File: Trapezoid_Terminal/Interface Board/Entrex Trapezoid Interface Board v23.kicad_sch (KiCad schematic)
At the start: 103 parts, among them P15 Conn_02x40_Odd_Even_Shielded, SW1 SW_DIP_x08

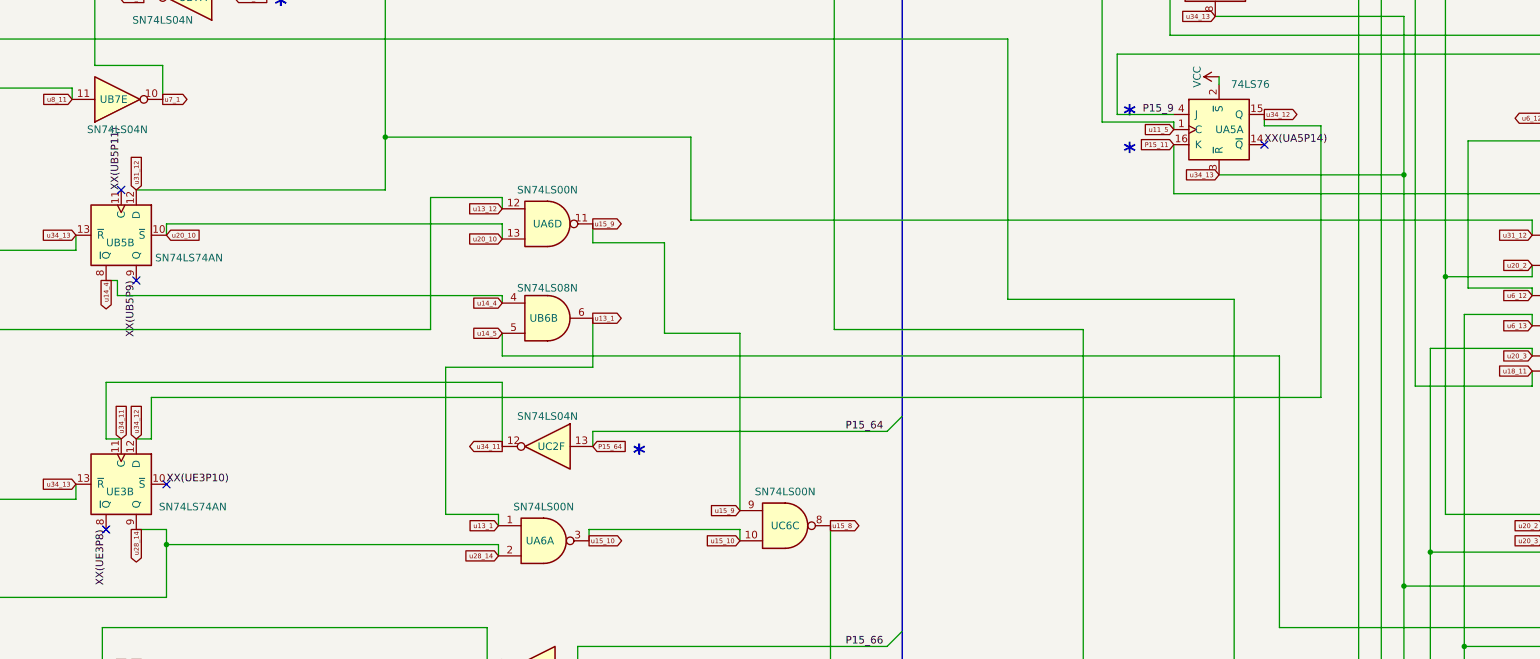
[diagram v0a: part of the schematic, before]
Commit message: UB5B Pin 11
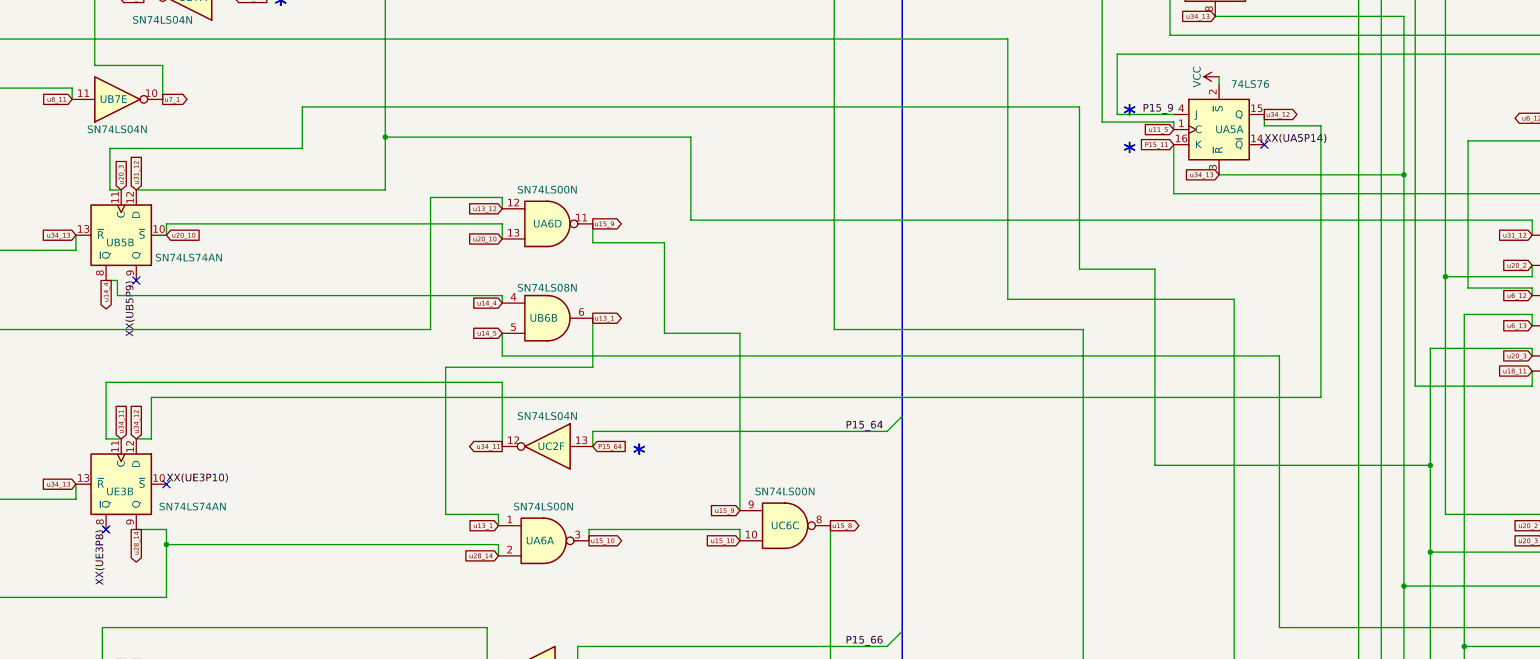
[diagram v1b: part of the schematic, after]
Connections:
- net XX(UB5P11) is gone; now on net u20_3: UB5.11 (C)
- no-connect marks 87 -> 86
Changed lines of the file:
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@@
   (junction (at 170.815 248.285) (diameter 0) (color 0 0 0 0)
   )
+  (junction (at 556.26 585.47) (diameter 0) (color 0 0 0 0)
+  )
   (junction (at 726.44 205.74) (diameter 0) (color 0 0 0 0)
   )
@@
   (no_connect (at 338.455 554.355))
   (no_connect (at 590.55 595.63))
-  (no_connect (at 335.915 539.115))
   (no_connect (at 582.93 590.55))
   (no_connect (at 711.2 173.99))
@@
     (stroke (width 0) (type default))
   )
+  (wire (pts (xy 509.905 552.45) (xy 509.905 585.47))
+    (stroke (width 0) (type default))
+  )
   (wire (pts (xy 400.05 567.055) (xy 530.86 567.055))
     (stroke (width 0) (type default))
@@
     (stroke (width 0) (type default))
   )
+  (wire (pts (xy 497.205 525.145) (xy 497.205 552.45))
+    (stroke (width 0) (type default))
+  )
   (wire (pts (xy 134.62 234.315) (xy 143.51 234.315))
     (stroke (width 0) (type default))
@@
     (stroke (width 0) (type default))
   )
+  (wire (pts (xy 334.01 539.115) (xy 334.01 532.13))
+    (stroke (width 0) (type default))
+  )
   (wire (pts (xy 561.975 615.95) (xy 615.315 615.95))
     (stroke (width 0) (type default))
@@
     (stroke (width 0) (type default))
   )
+  (wire (pts (xy 497.205 552.45) (xy 509.905 552.45))
+    (stroke (width 0) (type default))
+  )
   (wire (pts (xy 217.805 489.585) (xy 217.805 391.16))
     (stroke (width 0) (type default))
@@
     (stroke (width 0) (type default))
   )
+  (wire (pts (xy 334.01 532.13) (xy 366.395 532.13))
+    (stroke (width 0) (type default))
+  )
   (wire (pts (xy 1114.425 674.37) (xy 1110.615 674.37))
     (stroke (width 0) (type default))
@@
     (stroke (width 0) (type default))
   )
+  (wire (pts (xy 366.395 532.13) (xy 366.395 525.145))
+    (stroke (width 0) (type default))
+  )
   (wire (pts (xy 855.345 483.235) (xy 855.345 432.435))
     (stroke (width 0) (type default))
@@
     (stroke (width 0) (type default))
   )
+  (wire (pts (xy 509.905 585.47) (xy 556.26 585.47))
+    (stroke (width 0) (type default))
+  )
   (wire (pts (xy 317.5 160.02) (xy 363.22 160.02))
     (stroke (width 0) (type default))
@@
     (stroke (width 0) (type default))
   )
-  (wire (pts (xy 556.26 600.075) (xy 556.26 565.785))
+  (wire (pts (xy 556.26 600.075) (xy 556.26 585.47))
     (stroke (width 0) (type default))
   )
@@
     (stroke (width 0) (type default))
   )
+  (wire (pts (xy 366.395 525.145) (xy 497.205 525.145))
+    (stroke (width 0) (type default))
+  )
   (wire (pts (xy 387.985 450.85) (xy 363.855 450.85))
     (stroke (width 0) (type default))
@@
     (stroke (width 0) (type default))
   )
+  (wire (pts (xy 556.26 585.47) (xy 556.26 565.785))
+    (stroke (width 0) (type default))
+  )
   (wire (pts (xy 158.75 231.14) (xy 166.37 231.14))
     (stroke (width 0) (type default))
@@
     (stroke (width 0) (type default))
   )
+  (wire (pts (xy 335.915 539.115) (xy 334.01 539.115))
+    (stroke (width 0) (type default))
+  )
   (wire (pts (xy 407.67 222.25) (xy 407.67 220.345))
     (stroke (width 0) (type default))
@@
     (effects (font (size 1.27 1.27)) (justify left bottom))
   )
-  (label "XX(UB5P11)" (at 335.915 539.115 90) (fields_autoplaced)
-    (effects (font (size 1.27 1.27)) (justify left bottom))
-  )
   (label "XX(UC7P12)" (at 579.12 488.95 270) (fields_autoplaced)
     (effects (font (size 1.27 1.27)) (justify right bottom))
@@
     )
   )
+  (global_label "u20_3" (shape input) (at 335.915 539.115 90) (fields_autoplaced)
+    (effects (font (size 0.8 0.8)) (justify left))
+    (property "Intersheetrefs" "${INTERSHEET_REFS}" (at 335.915 533.6657 90)
+      (effects (font (size 1.27 1.27)) (justify left) hide)
+    )
+  )

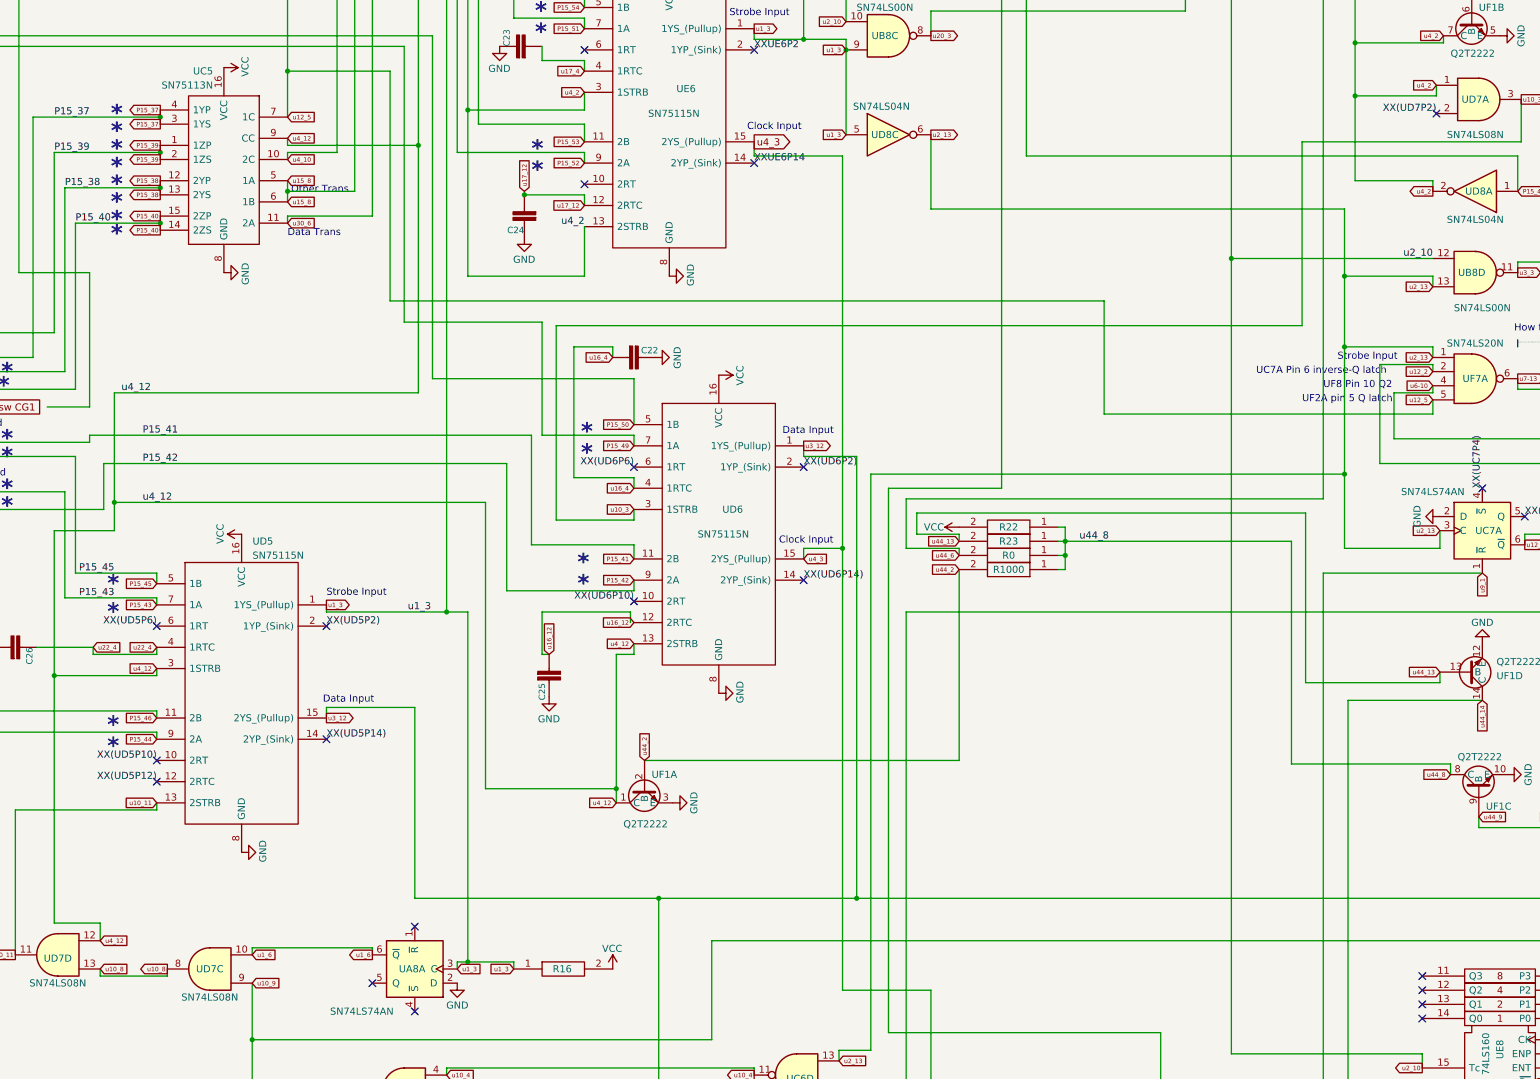
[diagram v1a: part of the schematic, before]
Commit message: Corrections & Testing
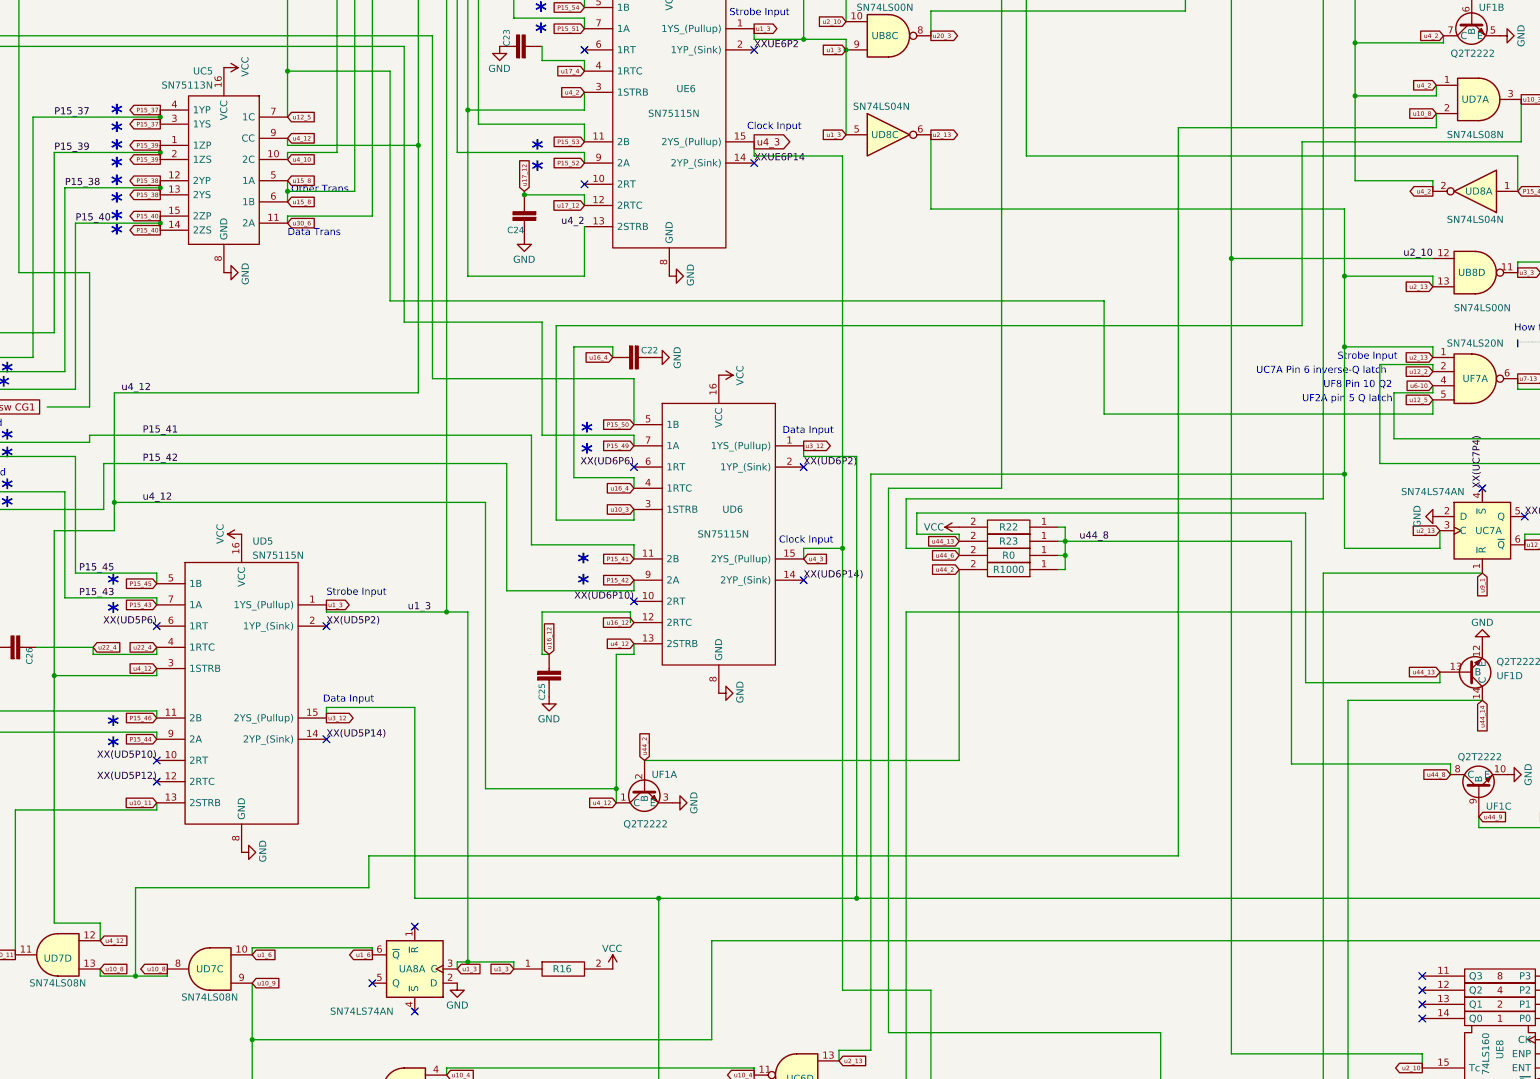
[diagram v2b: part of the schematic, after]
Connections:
- net XX(UD7P2) is gone; now on net u10_8: UD7.2
- no-connect marks 86 -> 85
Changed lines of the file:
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@@
   (junction (at 423.545 392.43) (diameter 0) (color 0 0 0 0)
   )
+  (junction (at 174.625 333.375) (diameter 0) (color 0 0 0 0)
+  )
   (junction (at 201.93 60.96) (diameter 0) (color 0 0 0 0)
   )
@@
   (no_connect (at 584.2 473.71))
   (no_connect (at 424.18 250.825))
-  (no_connect (at 408.305 178.435))
   (no_connect (at 739.775 264.795))
   (bus_entry (at 467.36 494.665) (size 2.54 2.54)
@@
     (stroke (width 0) (type default))
   )
+  (wire (pts (xy 361.95 180.975) (xy 408.305 180.975))
+    (stroke (width 0) (type default))
+  )
   (wire (pts (xy 169.545 657.86) (xy 169.545 659.13))
     (stroke (width 0) (type default))
@@
     (stroke (width 1) (type default))
   )
+  (wire (pts (xy 408.305 178.435) (xy 408.305 180.975))
+    (stroke (width 0) (type default))
+  )
   (wire (pts (xy 123.825 217.805) (xy 123.825 220.98))
     (stroke (width 0) (type default))
@@
     (stroke (width 0) (type default))
   )
+  (wire (pts (xy 174.625 317.5) (xy 216.535 317.5))
+    (stroke (width 0) (type default))
+  )
   (wire (pts (xy 748.665 463.55) (xy 788.035 463.55))
     (stroke (width 0) (type default))
@@
     (stroke (width 0) (type default))
   )
+  (wire (pts (xy 174.625 333.375) (xy 180.34 333.375))
+    (stroke (width 0) (type default))
+  )
   (wire (pts (xy 313.055 424.18) (xy 313.055 427.355))
     (stroke (width 0) (type default))
@@
     (stroke (width 0) (type default))
   )
+  (wire (pts (xy 216.535 317.5) (xy 216.535 311.785))
+    (stroke (width 0) (type default))
+  )
   (wire (pts (xy 225.425 135.255) (xy 225.425 184.15))
     (stroke (width 0) (type default))
@@
     (stroke (width 0) (type default))
   )
-  (wire (pts (xy 168.275 333.375) (xy 180.34 333.375))
+  (wire (pts (xy 168.275 333.375) (xy 174.625 333.375))
     (stroke (width 0) (type default))
   )
@@
     (stroke (width 1) (type default))
   )
+  (wire (pts (xy 174.625 333.375) (xy 174.625 317.5))
+    (stroke (width 0) (type default))
+  )
   (wire (pts (xy 156.845 66.04) (xy 156.845 67.31))
     (stroke (width 0) (type default))
@@
     (stroke (width 0) (type default))
   )
+  (wire (pts (xy 361.95 311.785) (xy 361.95 180.975))
+    (stroke (width 0) (type default))
+  )
   (wire (pts (xy 201.93 184.15) (xy 225.425 184.15))
     (stroke (width 0) (type default))
@@
     (stroke (width 1) (type default))
   )
+  (wire (pts (xy 216.535 311.785) (xy 361.95 311.785))
+    (stroke (width 0) (type default))
+  )
   (polyline (pts (xy 182.245 835.66) (xy 160.655 835.66))
     (stroke (width 0) (type default))
@@
     (effects (font (size 1.27 1.27)) (justify right bottom))
   )
-  (label "XX(UD7P2)" (at 408.305 178.435 180) (fields_autoplaced)
-    (effects (font (size 1.27 1.27)) (justify right bottom))
-  )
   (label "P15_40" (at 163.83 198.12 0) (fields_autoplaced)
     (effects (font (size 1.27 1.27)) (justify left bottom))
@@
     )
   )
+  (global_label "u10_8" (shape input) (at 408.305 178.435 180) (fields_autoplaced)
+    (effects (font (size 0.8 0.8)) (justify right))
+    (property "Intersheetrefs" "${INTERSHEET_REFS}" (at 402.8557 178.435 0)
+      (effects (font (size 1.27 1.27)) (justify right) hide)
+    )
+  )
